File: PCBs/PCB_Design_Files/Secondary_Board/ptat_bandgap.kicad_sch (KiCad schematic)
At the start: 15 parts, among them IC1 TLV2333IDGKR, Q1 DMMT3904W-7-F, Q2 DMMT3904W-7-F, U1 DMMT5401-7-F, U2 DMMT5401-7-F, U3 DMMT5401-7-F, U4 DMMT5401-7-F

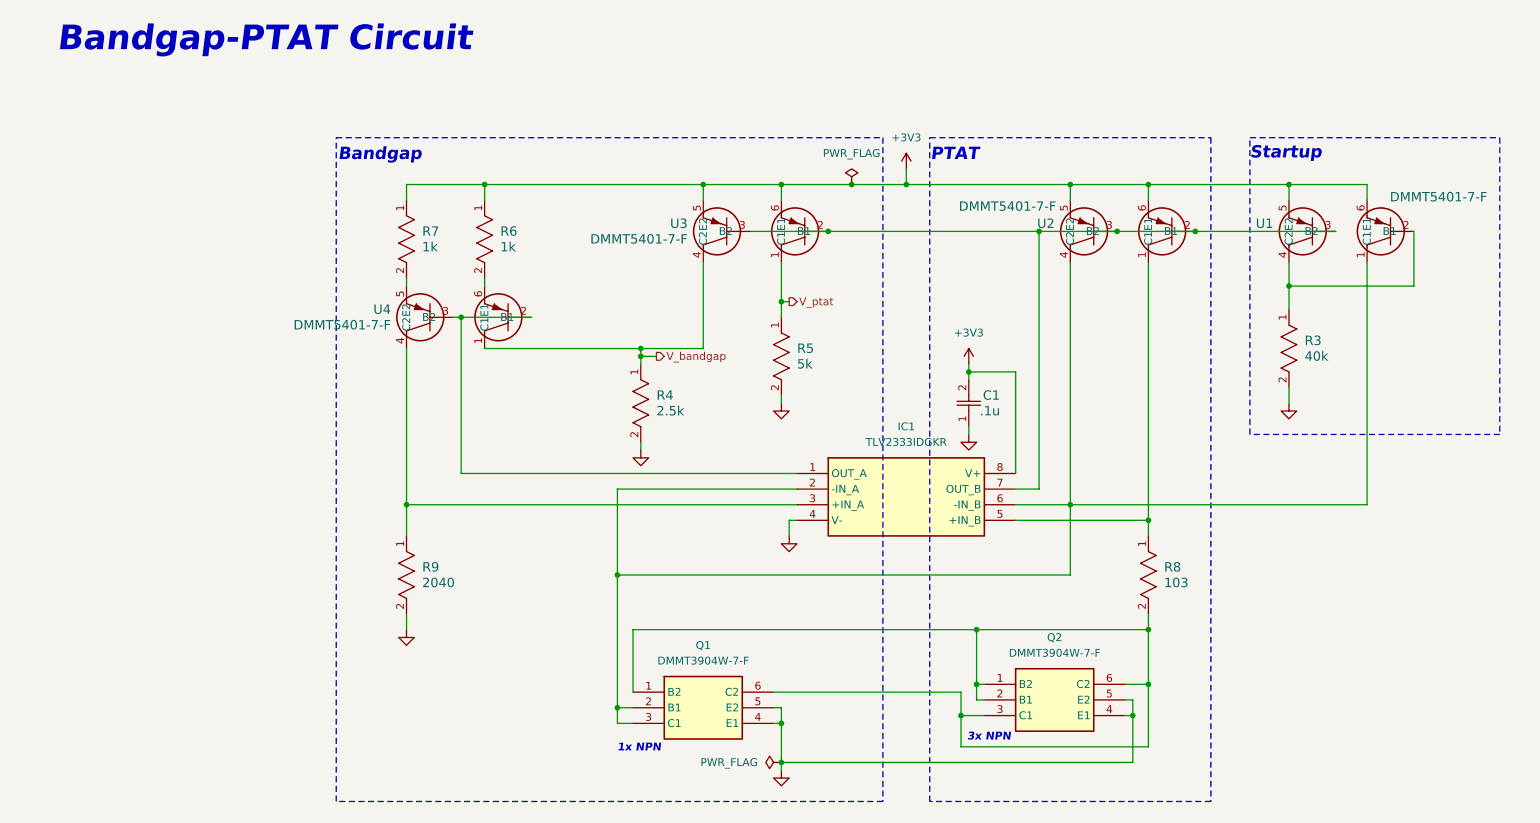
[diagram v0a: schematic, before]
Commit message: updated bg_ptat
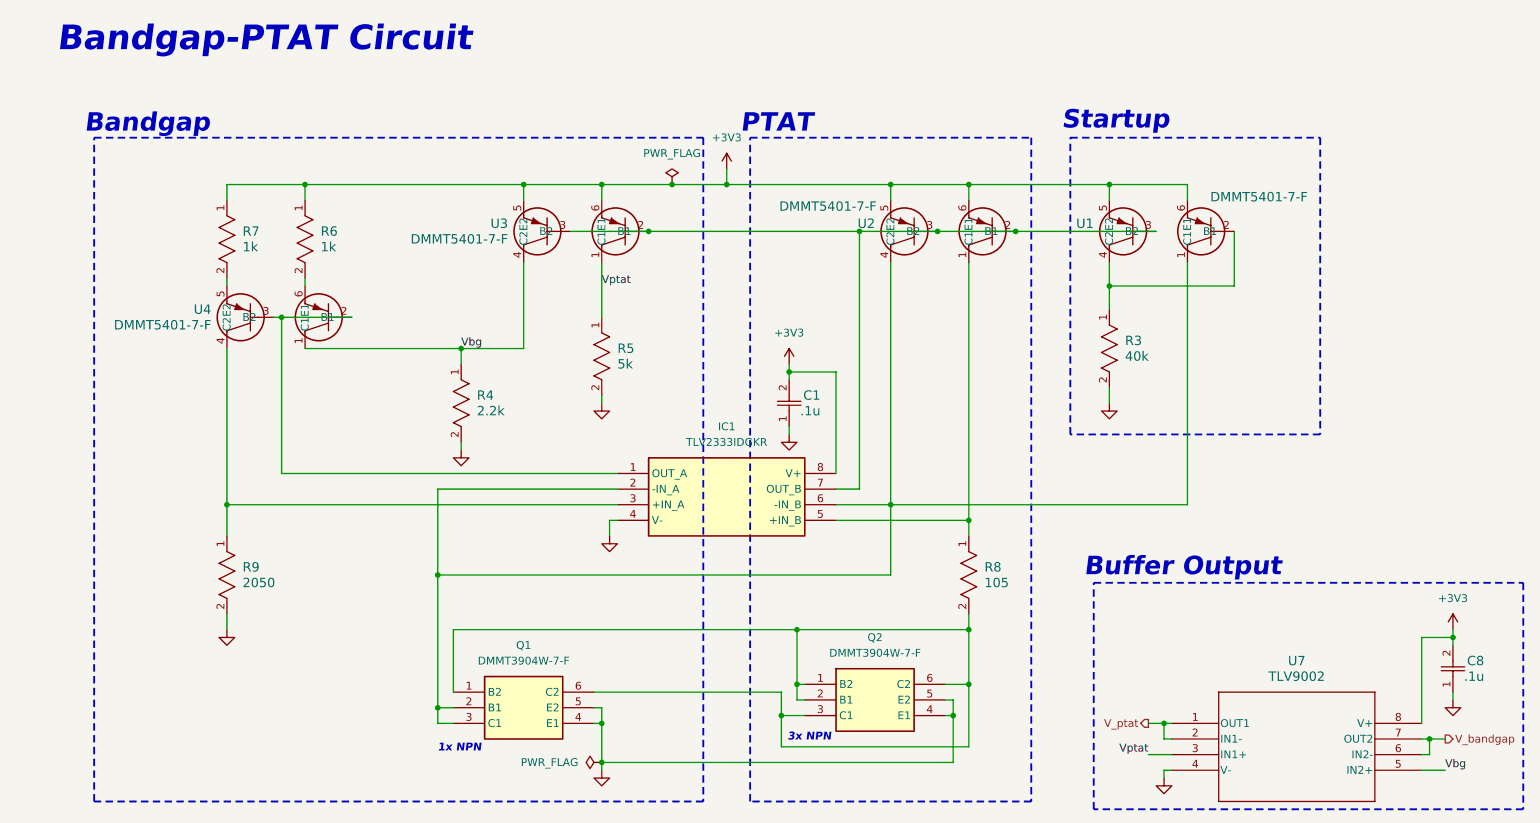
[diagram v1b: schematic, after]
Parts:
- added C8: .1u, Project Footprints:0603_capacitor, symbol Project_Symbols:0603_capacitor
- added U7: TLV9002, Project Footprints:TLV9002, symbol Project_Symbols:TLV9002
- R4: value 2.5k -> 2.2k
- R8: value 103 -> 105
- R9: value 2040 -> 2050
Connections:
- net +3V3: now also C8.2, U7.8 (V+)
- net GND: now also C8.1, U7.4 (V-)
- net V_bandgap: now also U7.6 (IN2-), U7.7 (OUT2); no longer R4.1, U3.4 (C2), U4.1 (C1)
- net V_ptat: now also U7.1 (OUT1), U7.2 (IN1-); no longer R5.1, U3.1 (C1)
- new net Vbg: R4.1, U3.4 (C2), U4.1 (C1), U7.5 (IN2+)
- new net Vptat: R5.1, U3.1 (C1), U7.3 (IN1+)
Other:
- note added: "Buffer Output"
- moved on the sheet: C1, IC1, Q1, Q2, R3, R4, R5, R6, R7, R8, R9, U1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
